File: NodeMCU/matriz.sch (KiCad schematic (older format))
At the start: 16 parts, among them Q1 Q_NPN_BCE, Q2 Q_NPN_BCE, Q3 Q_NPN_BCE, SW1 SW_Push_Open, U3 NodeMCU1.0(ESP-12E), U4 interfOut

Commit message: Esquematico testeado
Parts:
- removed U4: interfOut, symbol interfOut
- added J1: Conn_01x05, symbol Conn_01x05
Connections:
- net labels added: CLK, DOUT, GNDPWR, LD, V+
- wire segments 55 -> 59
- no-connect marks 23 -> 22
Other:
- moved on the sheet: Q1, R1, R2, SW1

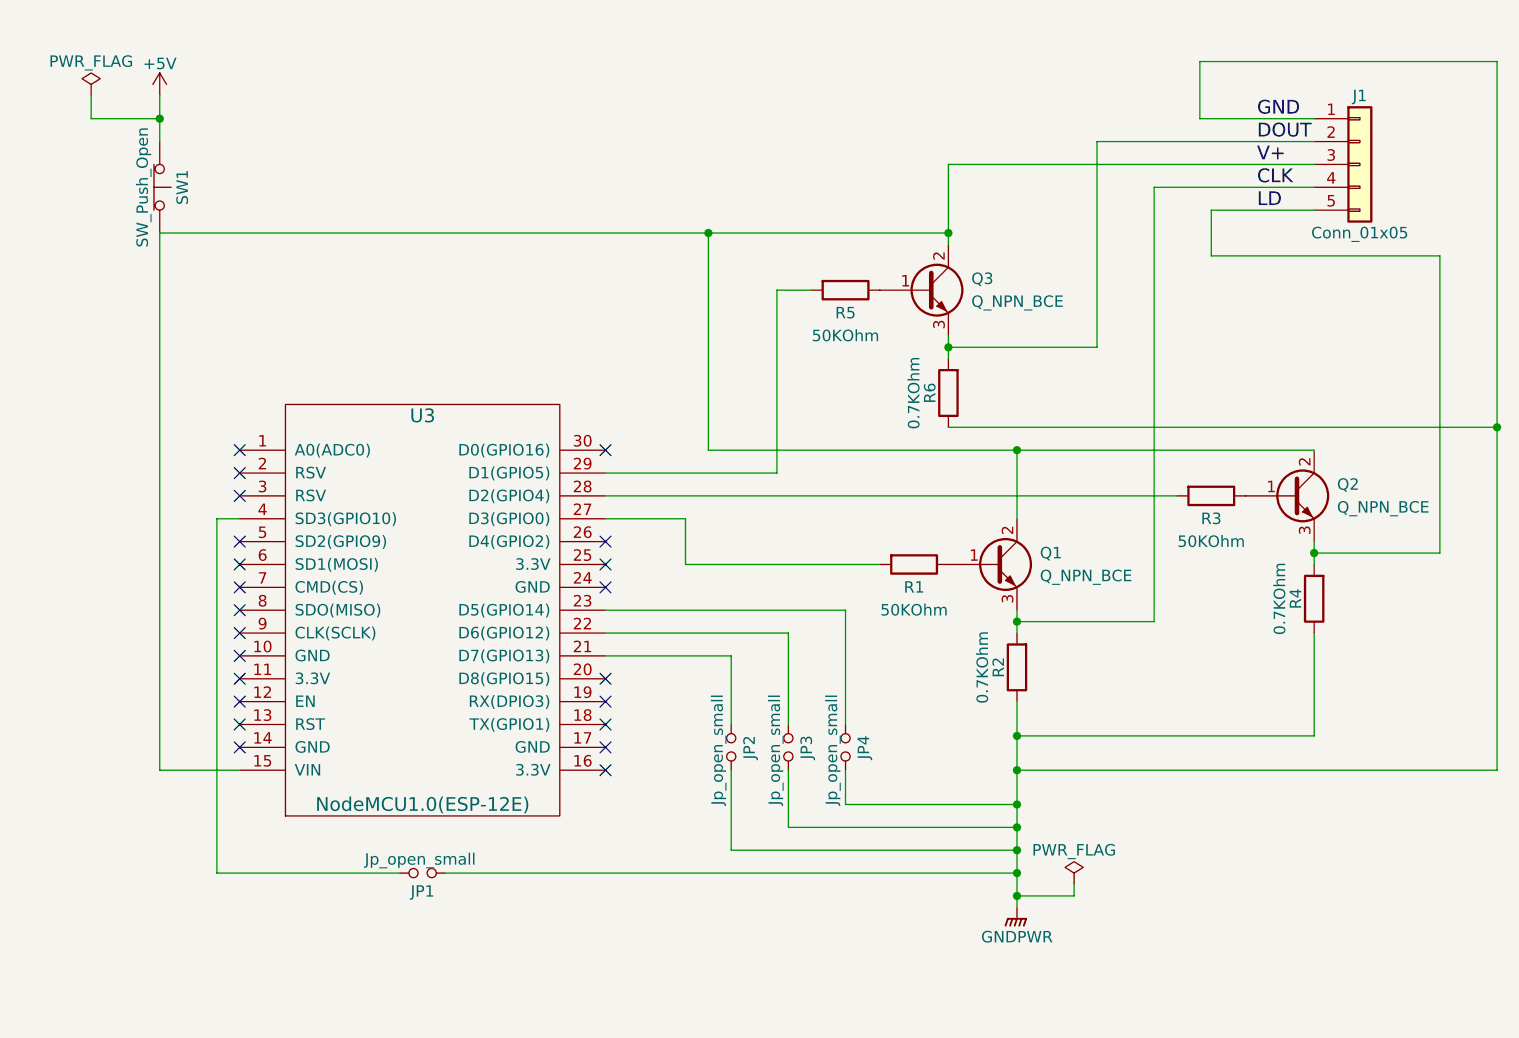
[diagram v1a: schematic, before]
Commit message: Footprint slave
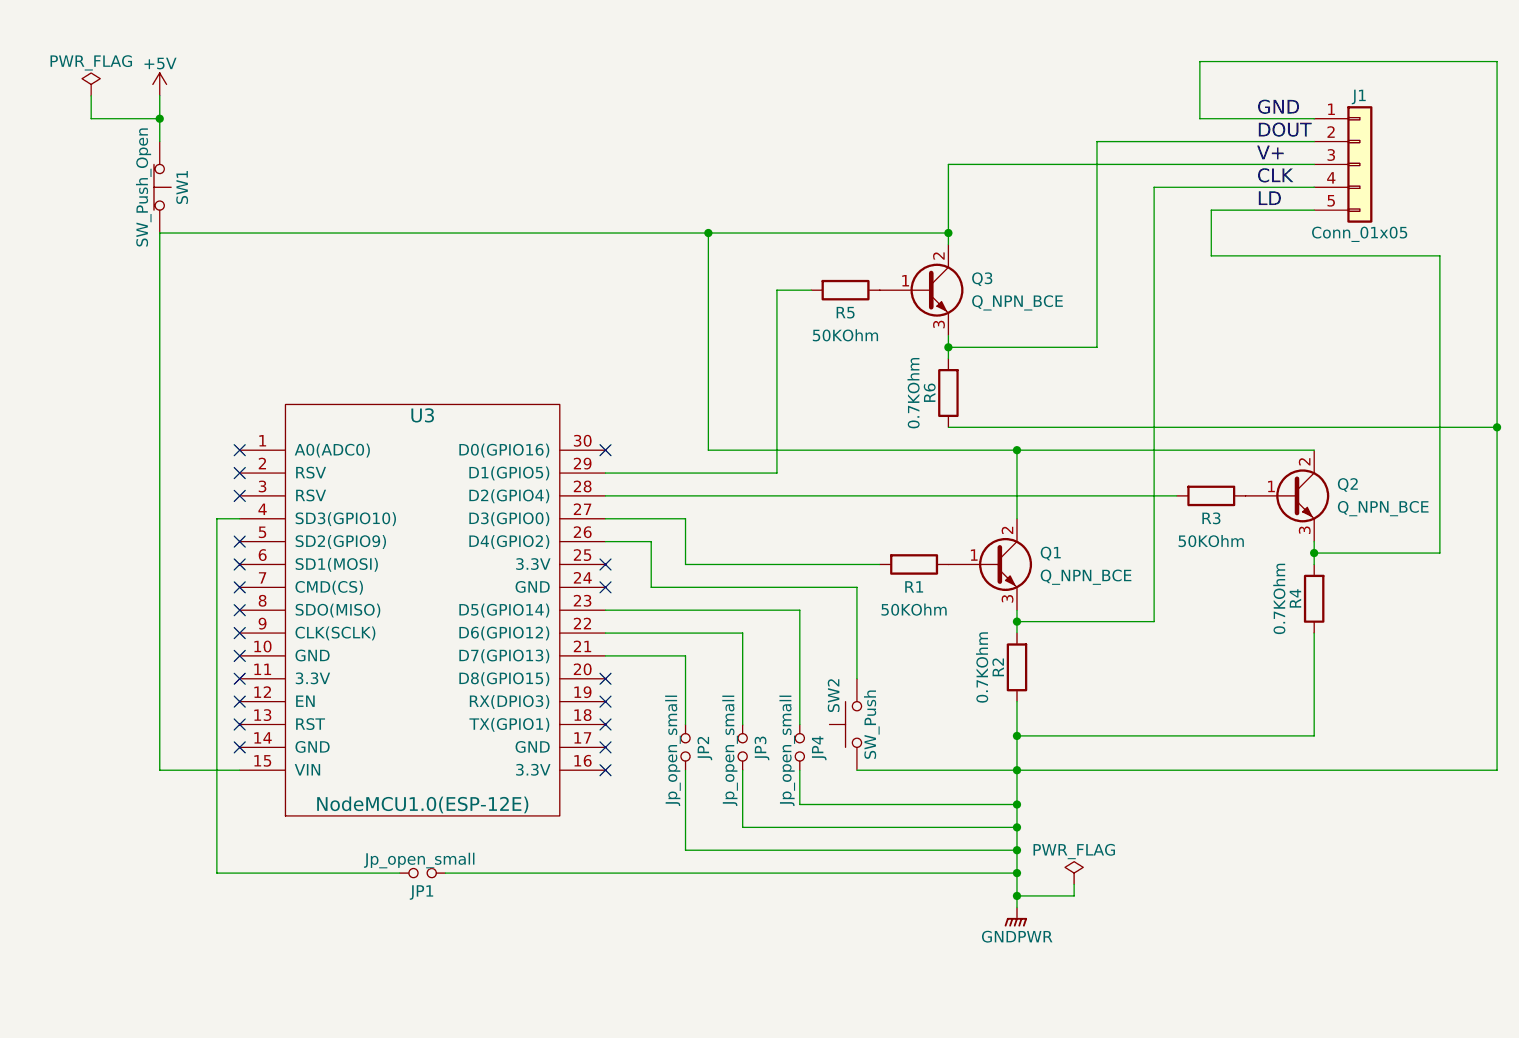
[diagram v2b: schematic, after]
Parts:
- added SW2: SW_Push, symbol SW_Push
- J1: footprint (none) -> Pin_Headers:Pin_Header_Angled_1x05_Pitch2.54mm
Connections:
- net GNDPWR: now also SW2.1
- net at U3.26 (D4(GPIO2)): now also SW2.2
- no-connect marks 22 -> 21
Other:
- moved on the sheet: JP2, JP3, JP4
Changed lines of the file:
@@
 F 0 "U3" H 4950 5750 60  0000 C CNN
 F 1 "NodeMCU1.0(ESP-12E)" H 4950 4050 60  0000 C CNN
-F 2 "" H 4350 4050 60  0000 C CNN
+F 2 "" H 4350 4050 60  0001 C CNN
 F 3 "" H 4350 4050 60  0000 C CNN
 	1    4950 4900
 	1    0    0    -1
 $EndComp
-NoConn ~ 5750 4600
 NoConn ~ 5750 4700
 NoConn ~ 5750 4800
@@
 L Jumper_NO_Small JP4
 U 1 1 5A08DDBF
-P 6800 5500
-F 0 "JP4" H 6800 5580 50  0000 C CNN
-F 1 "Jp_open_small" H 6810 5440 50  0000 C CNN
-F 2 "" H 6800 5500 50  0001 C CNN
-F 3 "" H 6800 5500 50  0001 C CNN
-	1    6800 5500
+P 6600 5500
+F 0 "JP4" H 6600 5580 50  0000 C CNN
+F 1 "Jp_open_small" H 6610 5440 50  0000 C CNN
+F 2 "" H 6600 5500 50  0001 C CNN
+F 3 "" H 6600 5500 50  0001 C CNN
+	1    6600 5500
 	0    1    1    0
 $EndComp
@@
 L Jumper_NO_Small JP3
 U 1 1 5A08DF42
-P 6550 5500
-F 0 "JP3" H 6550 5580 50  0000 C CNN
-F 1 "Jp_open_small" H 6560 5440 50  0000 C CNN
-F 2 "" H 6550 5500 50  0001 C CNN
-F 3 "" H 6550 5500 50  0001 C CNN
-	1    6550 5500
+P 6350 5500
+F 0 "JP3" H 6350 5580 50  0000 C CNN
+F 1 "Jp_open_small" H 6360 5440 50  0000 C CNN
+F 2 "" H 6350 5500 50  0001 C CNN
+F 3 "" H 6350 5500 50  0001 C CNN
+	1    6350 5500
 	0    1    1    0
 $EndComp
@@
 L Jumper_NO_Small JP2
 U 1 1 5A08DF95
-P 6300 5500
-F 0 "JP2" H 6300 5580 50  0000 C CNN
-F 1 "Jp_open_small" H 6310 5440 50  0000 C CNN
-F 2 "" H 6300 5500 50  0001 C CNN
-F 3 "" H 6300 5500 50  0001 C CNN
-	1    6300 5500
+P 6100 5500
+F 0 "JP2" H 6100 5580 50  0000 C CNN
+F 1 "Jp_open_small" H 6110 5440 50  0000 C CNN
+F 2 "" H 6100 5500 50  0001 C CNN
+F 3 "" H 6100 5500 50  0001 C CNN
+	1    6100 5500
 	0    1    1    0
 $EndComp
@@
 F 0 "J1" H 9050 3250 50  0000 C CNN
 F 1 "Conn_01x05" H 9050 2650 50  0000 C CNN
-F 2 "" H 9050 2950 50  0001 C CNN
+F 2 "Pin_Headers:Pin_Header_Angled_1x05_Pitch2.54mm" H 9050 2950 50  0001 C CNN
 F 3 "" H 9050 2950 50  0001 C CNN
 	1    9050 2950
@@
 	7250 2950 8850 2950
 Wire Wire Line
-	9650 2500 9650 5600
+	9650 5600 9650 2500
 Wire Wire Line
 	9650 2500 8350 2500
@@
 	8350 2750 8850 2750
 Wire Wire Line
-	6800 5600 6800 5750
-Wire Wire Line
-	6550 5600 6550 5850
-Wire Wire Line
-	6300 5600 6300 5950
-Wire Wire Line
-	5750 4900 6800 4900
-Wire Wire Line
-	5750 5000 6550 5000
-Wire Wire Line
-	5750 5100 6300 5100
-Wire Wire Line
-	6800 4900 6800 5400
-Wire Wire Line
-	6300 5100 6300 5400
-Wire Wire Line
-	6550 5000 6550 5400
+	6600 5600 6600 5750
+Wire Wire Line
+	6350 5600 6350 5850
+Wire Wire Line
+	6100 5600 6100 5950
+Wire Wire Line
+	6600 4900 6600 5400
+Wire Wire Line
+	6100 5100 6100 5400
+Wire Wire Line
+	6350 5000 6350 5400
 Wire Wire Line
 	3800 2750 3500 2750
@@
 	7550 5300 7550 6200
 Wire Wire Line
-	6300 5950 7550 5950
+	6100 5950 7550 5950
 Connection ~ 7550 5950
 Wire Wire Line
-	6550 5850 7550 5850
-Wire Wire Line
-	6800 5750 7550 5750
+	6350 5850 7550 5850
+Wire Wire Line
+	6600 5750 7550 5750
 Connection ~ 7550 5850
 Connection ~ 7550 5750
@@
 Connection ~ 7250 3250
 Wire Wire Line
-	9650 5600 7550 5600
+	6850 5600 9650 5600
 Connection ~ 7550 5600
 Wire Wire Line
@@
 Wire Wire Line
 	3800 5600 3800 3250
+Wire Wire Line
+	6600 4900 5750 4900
+Wire Wire Line
+	6350 5000 5750 5000
+Wire Wire Line
+	6100 5100 5750 5100
+$Comp
+L SW_Push SW2
+U 1 1 5A121D29
+P 6850 5400
+F 0 "SW2" H 6900 5500 50  0000 L CNN
+F 1 "SW_Push" H 6850 5340 50  0000 C CNN
+F 2 "" H 6850 5600 50  0001 C CNN
+F 3 "" H 6850 5600 50  0001 C CNN
+	1    6850 5400
+	0    -1   -1   0
+$EndComp
+Wire Wire Line
+	5750 4600 5950 4600
+Wire Wire Line
+	5950 4600 5950 4800
+Wire Wire Line
+	5950 4800 6850 4800
+Wire Wire Line
+	6850 4800 6850 5200
 $EndSCHEMATC

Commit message: master changes
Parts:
- JP1, JP2, JP3, JP4, SW1, SW2: footprint (none) -> Connectors:PINHEAD1-2
- Q1, Q2, Q3: footprint (none) -> Transistors_OldSowjetAera:OldSowjetaera_Transistor_Type-II_BigPads
- R1, R2, R3, R4, R5, R6: footprint (none) -> Resistors_THT:R_Axial_DIN0207_L6.3mm_D2.5mm_P7.62mm_Horizontal
- U3: footprint (none) -> NodeMCU:NodeMCU1.0(12-E)
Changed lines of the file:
@@
 F 0 "U3" H 4950 5750 60  0000 C CNN
 F 1 "NodeMCU1.0(ESP-12E)" H 4950 4050 60  0000 C CNN
-F 2 "" H 4350 4050 60  0001 C CNN
+F 2 "NodeMCU:NodeMCU1.0(12-E)" H 4350 4050 60  0001 C CNN
 F 3 "" H 4350 4050 60  0000 C CNN
 	1    4950 4900
@@
 F 0 "SW1" H 3800 3150 50  0000 C CNN
 F 1 "SW_Push_Open" H 3800 2975 50  0000 C CNN
-F 2 "" H 3800 3250 50  0001 C CNN
+F 2 "Connectors:PINHEAD1-2" H 3800 3250 50  0001 C CNN
 F 3 "" H 3800 3250 50  0001 C CNN
 	1    3800 3050
@@
 F 0 "JP4" H 6600 5580 50  0000 C CNN
 F 1 "Jp_open_small" H 6610 5440 50  0000 C CNN
-F 2 "" H 6600 5500 50  0001 C CNN
+F 2 "Connectors:PINHEAD1-2" H 6600 5500 50  0001 C CNN
 F 3 "" H 6600 5500 50  0001 C CNN
 	1    6600 5500
@@
 F 0 "JP3" H 6350 5580 50  0000 C CNN
 F 1 "Jp_open_small" H 6360 5440 50  0000 C CNN
-F 2 "" H 6350 5500 50  0001 C CNN
+F 2 "Connectors:PINHEAD1-2" H 6350 5500 50  0001 C CNN
 F 3 "" H 6350 5500 50  0001 C CNN
 	1    6350 5500
@@
 F 0 "JP2" H 6100 5580 50  0000 C CNN
 F 1 "Jp_open_small" H 6110 5440 50  0000 C CNN
-F 2 "" H 6100 5500 50  0001 C CNN
+F 2 "Connectors:PINHEAD1-2" H 6100 5500 50  0001 C CNN
 F 3 "" H 6100 5500 50  0001 C CNN
 	1    6100 5500
@@
 F 0 "JP1" H 4950 6130 50  0000 C CNN
 F 1 "Jp_open_small" H 4960 5990 50  0000 C CNN
-F 2 "" H 4950 6050 50  0001 C CNN
+F 2 "Connectors:PINHEAD1-2" H 4950 6050 50  0001 C CNN
 F 3 "" H 4950 6050 50  0001 C CNN
 	1    4950 6050
@@
 F 0 "R1" V 7200 4700 50  0000 C CNN
 F 1 "50KOhm" V 7300 4700 50  0000 C CNN
-F 2 "" V 7030 4700 50  0001 C CNN
+F 2 "Resistors_THT:R_Axial_DIN0207_L6.3mm_D2.5mm_P7.62mm_Horizontal" V 7030 4700 50  0001 C CNN
 F 3 "" H 7100 4700 50  0001 C CNN
 	1    7100 4700
@@
 F 0 "R2" V 7630 5150 50  0000 C CNN
 F 1 "0.7KOhm" V 7700 5150 50  0000 C CNN
-F 2 "" V 7480 5150 50  0001 C CNN
+F 2 "Resistors_THT:R_Axial_DIN0207_L6.3mm_D2.5mm_P7.62mm_Horizontal" V 7480 5150 50  0001 C CNN
 F 3 "" H 7550 5150 50  0001 C CNN
 	1    7550 5150
@@
 F 0 "Q1" H 7650 4750 50  0000 L CNN
 F 1 "Q_NPN_BCE" H 7650 4650 50  0000 L CNN
-F 2 "" H 7650 4800 50  0001 C CNN
+F 2 "Transistors_OldSowjetAera:OldSowjetaera_Transistor_Type-II_BigPads" H 7650 4800 50  0001 C CNN
 F 3 "" H 7450 4700 50  0001 C CNN
 	1    7450 4700
@@
 F 0 "R3" V 8500 4400 50  0000 C CNN
 F 1 "50KOhm" V 8600 4400 50  0000 C CNN
-F 2 "" V 8330 4400 50  0001 C CNN
+F 2 "Resistors_THT:R_Axial_DIN0207_L6.3mm_D2.5mm_P7.62mm_Horizontal" V 8330 4400 50  0001 C CNN
 F 3 "" H 8400 4400 50  0001 C CNN
 	1    8400 4400
@@
 F 0 "R4" V 8930 4850 50  0000 C CNN
 F 1 "0.7KOhm" V 9000 4850 50  0000 C CNN
-F 2 "" V 8780 4850 50  0001 C CNN
+F 2 "Resistors_THT:R_Axial_DIN0207_L6.3mm_D2.5mm_P7.62mm_Horizontal" V 8780 4850 50  0001 C CNN
 F 3 "" H 8850 4850 50  0001 C CNN
 	1    8850 4850
@@
 F 0 "Q2" H 8950 4450 50  0000 L CNN
 F 1 "Q_NPN_BCE" H 8950 4350 50  0000 L CNN
-F 2 "" H 8950 4500 50  0001 C CNN
+F 2 "Transistors_OldSowjetAera:OldSowjetaera_Transistor_Type-II_BigPads" H 8950 4500 50  0001 C CNN
 F 3 "" H 8750 4400 50  0001 C CNN
 	1    8750 4400
@@
 F 0 "R5" V 6900 3500 50  0000 C CNN
 F 1 "50KOhm" V 7000 3500 50  0000 C CNN
-F 2 "" V 6730 3500 50  0001 C CNN
+F 2 "Resistors_THT:R_Axial_DIN0207_L6.3mm_D2.5mm_P7.62mm_Horizontal" V 6730 3500 50  0001 C CNN
 F 3 "" H 6800 3500 50  0001 C CNN
 	1    6800 3500
@@
 F 0 "R6" V 7330 3950 50  0000 C CNN
 F 1 "0.7KOhm" V 7400 3950 50  0000 C CNN
-F 2 "" V 7180 3950 50  0001 C CNN
+F 2 "Resistors_THT:R_Axial_DIN0207_L6.3mm_D2.5mm_P7.62mm_Horizontal" V 7180 3950 50  0001 C CNN
 F 3 "" H 7250 3950 50  0001 C CNN
 	1    7250 3950
@@
 F 0 "Q3" H 7350 3550 50  0000 L CNN
 F 1 "Q_NPN_BCE" H 7350 3450 50  0000 L CNN
-F 2 "" H 7350 3600 50  0001 C CNN
+F 2 "Transistors_OldSowjetAera:OldSowjetaera_Transistor_Type-II_BigPads" H 7350 3600 50  0001 C CNN
 F 3 "" H 7150 3500 50  0001 C CNN
 	1    7150 3500
@@
 F 0 "SW2" H 6900 5500 50  0000 L CNN
 F 1 "SW_Push" H 6850 5340 50  0000 C CNN
-F 2 "" H 6850 5600 50  0001 C CNN
+F 2 "Connectors:PINHEAD1-2" H 6850 5600 50  0001 C CNN
 F 3 "" H 6850 5600 50  0001 C CNN
 	1    6850 5400
